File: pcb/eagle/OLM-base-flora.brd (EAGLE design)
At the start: 100 x 80 mm, 54 parts, among them CN1 MiniB USB, IC1 ATMEGA32U4-AU, IC2 LP2985-3.3v, IC3 DS1307, IC6 ENC28J60, T1 IRLML2246, U2 USD-SOCKETMICRO-SD-SOCKET-TAO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, X1 32.657k, X2A 25MHz, X2A1 25MHz, X3 8MHz

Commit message: added some details
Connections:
- removed net D0: U2.2
- removed net SCL: IC3.6, RCL.2
- removed net SDA: IC3.5, RDA.2
- net D2/SDA: now also IC3.5, RDA.2
- net D3/SCL: now also IC3.6, RCL.2
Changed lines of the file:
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@@
 <contactref element="IC1" pad="41"/>
-</signal>
-<signal name="D0">
-<contactref element="U2" pad="2"/>
 </signal>
 <signal name="RESET">
@@
 <contactref element="IC6" pad="9"/>
 </signal>
-<signal name="SDA">
-<contactref element="IC3" pad="5"/>
-<contactref element="RDA" pad="2"/>
-<wire x1="66.7766" y1="33.655" x2="66.99" y2="48.26" width="0" layer="19" extent="1-1"/>
-</signal>
-<signal name="SCL">
-<contactref element="IC3" pad="6"/>
-<contactref element="RCL" pad="2"/>
-<wire x1="66.7766" y1="32.385" x2="72.07" y2="40.64" width="0" layer="19" extent="1-1"/>
-</signal>
 <signal name="N$36">
 <contactref element="IC3" pad="3"/>
@@
 <signal name="D2/SDA">
 <contactref element="IC1" pad="19"/>
+<contactref element="IC3" pad="5"/>
+<contactref element="RDA" pad="2"/>
+<wire x1="66.99" y1="48.26" x2="81.61" y2="47.54" width="0" layer="19" extent="1-1"/>
+<wire x1="66.7766" y1="33.655" x2="66.99" y2="48.26" width="0" layer="19" extent="1-1"/>
 </signal>
 <signal name="D3/SCL">
 <contactref element="IC1" pad="18"/>
+<contactref element="IC3" pad="6"/>
+<contactref element="RCL" pad="2"/>
+<wire x1="72.07" y1="40.64" x2="80.81" y2="47.54" width="0" layer="19" extent="1-1"/>
+<wire x1="66.7766" y1="32.385" x2="72.07" y2="40.64" width="0" layer="19" extent="1-1"/>
 </signal>
 <signal name="D4/A6">

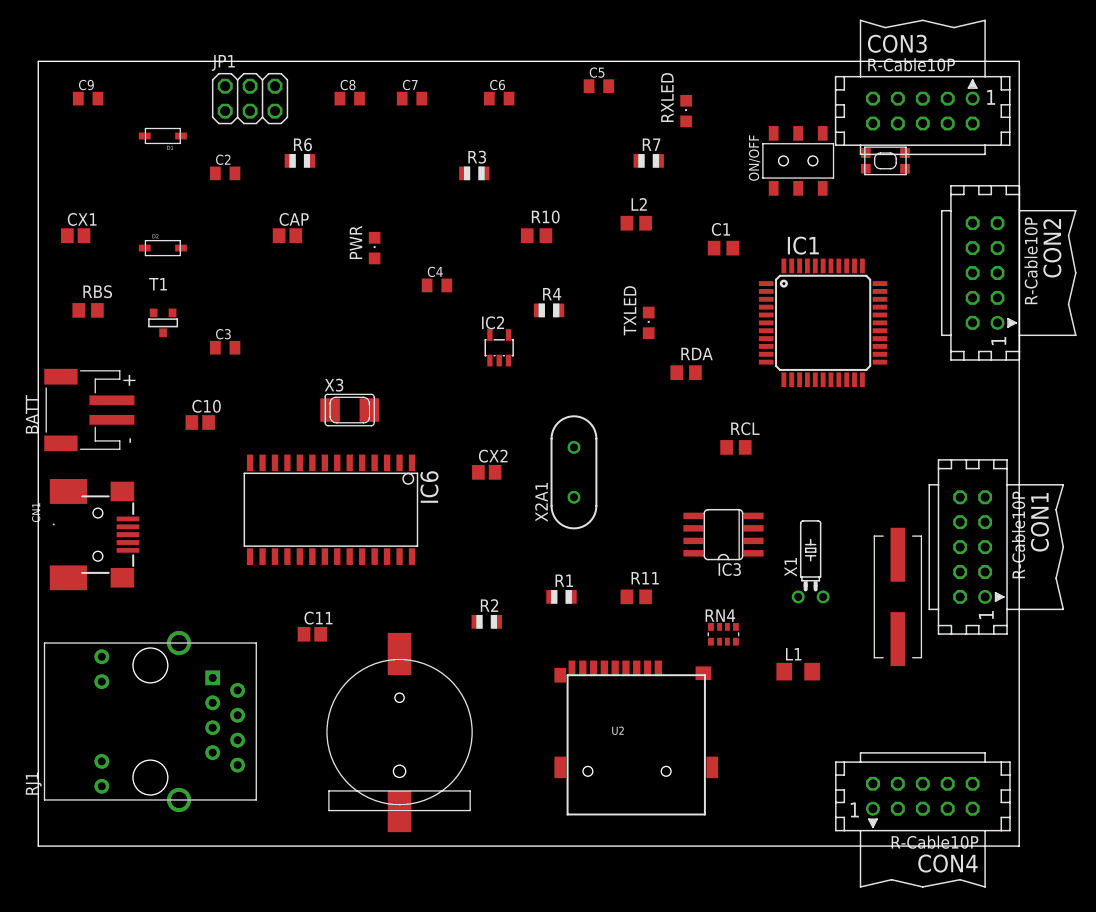
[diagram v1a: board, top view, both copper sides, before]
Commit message: made some changes
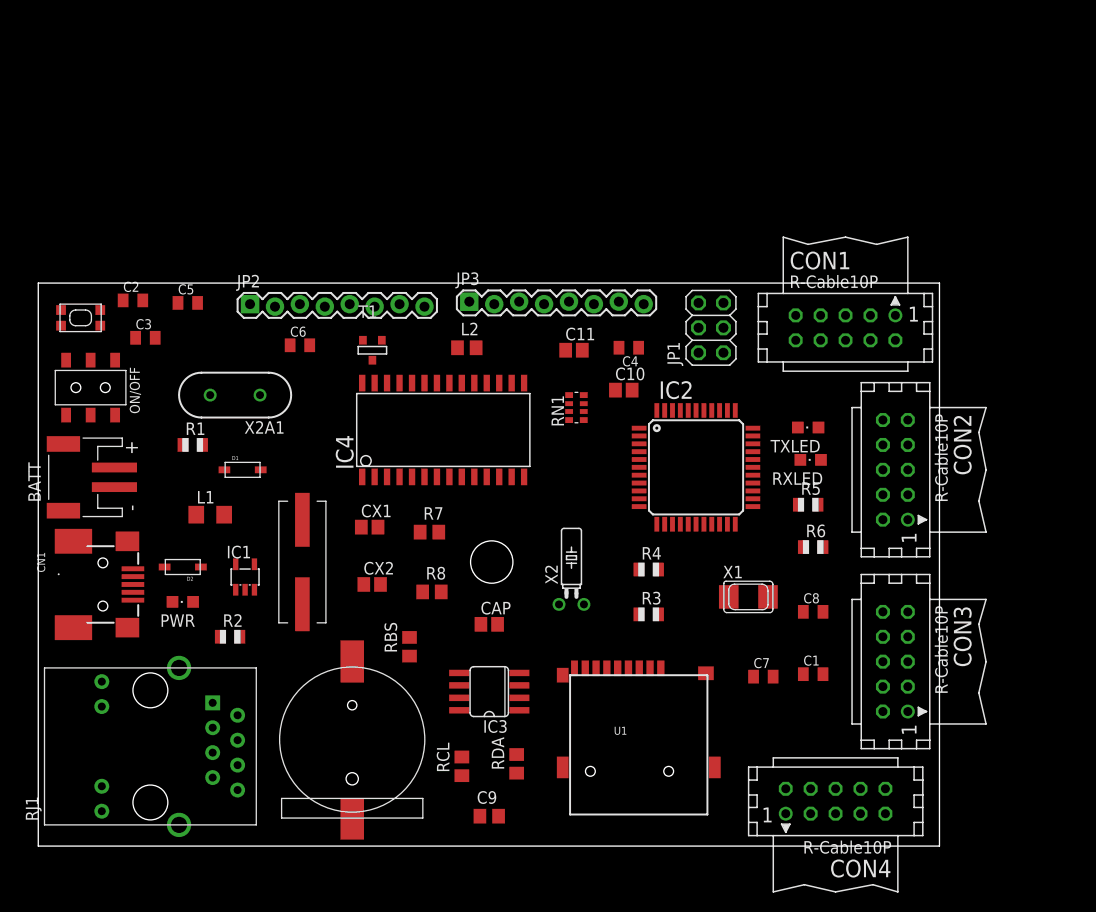
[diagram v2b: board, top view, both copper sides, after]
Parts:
- removed IC6: ENC28J60, SparkFun:SOIC28WLONG
- removed R10, R11: 330, rcl:R0805
- removed RN4: 49.9, resistor-dil:EXB38V
- removed U2: USD-SOCKETMICRO-SD-SOCKET-TAOBAO, SparkFunNew:MICRO-SD-SOCKET-TAOBAO
- removed X3: 8MHz, adaprog:NX5032
- added IC4: ENC28J60, SparkFun:SOIC28WLONG
- added JP2, JP3: (no value), SparkFun-Connectors:1X08_LOCK
- added R5: 1K, adafruit:R0805
- added R8: 330, rcl:R0805
- added RN1: 49.9, resistor-dil:EXB38V
- added U1: USD-SOCKETMICRO-SD-SOCKET-TAOBAO, SparkFunNew:MICRO-SD-SOCKET-TAOBAO
- added X2: 32.657k, crystal:TC26H
- C1: value 0.1u -> 10uF; device rcl:C0805 -> adafruit:C0805K
- C2, C3: value 18pF -> 10uF
- C7, C8: value 10uF -> 18pF
- C9: value 10uF -> 0.1u; device adafruit:C0805K -> rcl:C0805
- IC1: value ATMEGA32U4-AU -> LP2985-3.3v; device adaprog:TQFP44 -> adafruit:SOT23-5L
- IC2: value LP2985-3.3v -> ATMEGA32U4-AU; device adafruit:SOT23-5L -> adaprog:TQFP44
- R1: value 22 -> 10K
- R2: value 22 -> 470
- R3: value 470 -> 22
- R4: value 1K -> 22
- R7: value 10K -> 330; device adafruit:R0805 -> rcl:R0805
- X1: value 32.657k -> 8MHz; device crystal:TC26H -> adaprog:NX5032
- moved C9 83.8 mm to (46.0, 3.05)
- moved BOOT 83.6 mm to (4.32, 53.8)
- moved ON/OFF 75.7 mm to (5.33, 46.7), turned to 180 degrees
- moved C8 70.5 mm to (79.0, 23.9)
- moved C7 69.0 mm to (73.9, 17.3)
- moved R6 65.5 mm to (79.0, 30.5)
- moved IC1 64.4 mm to (21.1, 27.4)
- moved L1 62.0 mm to (17.5, 33.8)
- moved X2A 60.8 mm to (26.9, 29.0)
- moved CON3 56.2 mm to (87.4, 18.8), turned to 270 degrees
- moved JP1 52.5 mm to (68.6, 52.8), turned to 90 degrees
- moved R3 48.3 mm to (62.2, 23.6)
- moved RBS 47.4 mm to (37.8, 20.3), turned to 90 degrees
- moved C5 47.4 mm to (15.2, 55.4)
- moved CAP 44.6 mm to (46.0, 22.6)
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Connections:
- removed net AIO: CON1.4, CON2.4, CON3.4, CON4.4
- removed net DIO1: CON1.8, CON2.8, CON3.8, CON4.8
- removed net DIO2: CON1.9, CON2.9, CON3.9, CON4.9
- removed net DIO3: CON1.7, CON2.7, CON3.7, CON4.7
- new net A4/SDA: JP2.8
- new net A5/SCL: JP2.7
- new net D2: JP2.4
- new net D3/PWM: JP2.3
- new net E-CLK: JP2.6
- new net E-INT: JP2.5
- net +3V3: now also C2.1, C3.1, C4.1, C9.1, CON1.6, CON2.6, CON3.6, CON4.6, IC1.5, IC2.14, IC2.24, IC2.34, IC2.42, IC2.44, IC2.6, IC4.15, IC4.19, IC4.20, IC4.25, IC4.28, R2.2, U1.4; no longer C1.1, C6.1, C7.1, C8.1, IC1.14, IC1.24, IC1.34, IC1.42, IC1.44, IC1.6, IC2.5, IC6.15, IC6.19, IC6.20, IC6.25, IC6.28, R3.2, U2.4
- net +5V: now also C1.1, D2.A, IC2.7; no longer C9.1, D1.A, IC1.7
- net A0: now also CON1.4, CON3.4, IC2.36; no longer IC1.36
- net A1: now also CON1.2, CON3.2, IC2.37; no longer IC1.37
- net A2: now also CON2.4, CON4.4, IC2.38; no longer IC1.38
- net A3: now also CON2.2, CON4.2, IC2.39; no longer IC1.39
- net A4: now also IC2.40; no longer IC1.40
- net A5: now also IC2.41; no longer IC1.41
- net D0/RX: now also IC2.20, JP3.5; no longer IC1.20
- net D1/TX: now also IC2.21, JP3.4; no longer IC1.21
- net D2/SDA: now also IC2.19; no longer IC1.19
- net D3/SCL: now also IC2.18; no longer IC1.18
- net D4: now also IC4.9; no longer IC6.9
- net D4/A6: now also IC2.25; no longer IC1.25
- net D5*: now also CON1.9, CON3.9, IC2.31; no longer IC1.31
- net D6*/A8: now also IC2.27; no longer IC1.27
- net D7/AIN0: now also IC2.1; no longer IC1.1
- net GND: now also CON1.8, CON2.8, CON3.8, CON4.8, IC1.2, IC2.15, IC2.23, IC2.33, IC2.35, IC2.43, IC2.5, IC4.11, IC4.18, IC4.2, IC4.21, IC4.22, JP2.1, JP3.6, R5.2, U1.6; no longer CON1.6, CON2.6, CON3.6, CON4.6, IC1.15, IC1.23, IC1.33, IC1.35, IC1.43, IC1.5, IC2.2, IC6.11, IC6.18, IC6.2, IC6.21, IC6.22, R4.2, U2.6
- net IO10*/A11: now also CON1.7, CON3.7, IC2.30; no longer IC1.30
- net IO11*: now also IC2.12; no longer IC1.12
- net IO12*/A7: now also IC2.26; no longer IC1.26
- net IO13*: now also IC2.32; no longer IC1.32
- net IO8/A9: now also CON2.9, CON4.9, IC2.28; no longer IC1.28
- net IO9*/A10: now also CON2.7, CON4.7, IC2.29; no longer IC1.29
- net LEDA: now also R7.2; no longer R10.2
- net LEDB: now also R8.2; no longer R11.2
- net MISO: now also IC2.11, IC4.6, U1.7; no longer IC1.11, IC6.6, U2.7
- net MISO/D12: now also JP3.2
- net MOSI: now also IC2.10, IC4.7, U1.3; no longer IC1.10, IC6.7, U2.3
- net MOSI/D11: now also JP3.3
- net N$1: now also R2.1; no longer R3.1
- net N$11: now also R5.1; no longer R4.1
- net N$13: now also R1.1; no longer R7.1
- net N$2: now also R3.1; no longer R2.1
- net N$3: now also IC2.3, R4.2; no longer IC1.3, R1.2
- net N$34: now also IC4.27, R7.1; no longer IC6.27, R10.1
- net N$37: now also IC4.26, R8.1; no longer IC6.26, R11.1
- net N$39: now also IC4.1; no longer IC6.1
- net N$4: now also IC2.4, R3.2; no longer IC1.4, R2.2
- net N$41: now also IC4.24; no longer IC6.24
- net N$42: now also IC4.23; no longer IC6.23
- net N$47: now also X2.1; no longer X1.1
- net N$5: now also R4.1; no longer R1.1
- net N$50: now also X2.2; no longer X1.2
- net N$54: now also C10.2, RN1.5, RN1.6; no longer C11.2, RN4.5, RN4.6
- net N$59: now also IC4.14; no longer IC6.14
- net N$6: now also D1.C, R1.2; no longer D2.C, R7.2
- net N$7: now also D1.A; no longer D2.A
- net N$8: now also C7.1, IC2.17, X1.P$2; no longer C2.1, IC1.17, X3.P$2
- net N$9: now also C8.1, IC2.16, X1.P$1; no longer C3.1, IC1.16, X3.P$1
- net RD+: now also IC4.13, RN1.4; no longer IC6.13, RN4.4
- net RD-: now also IC4.12, RN1.3; no longer IC6.12, RN4.3
- net RESET: now also IC4.10; no longer IC6.10
- net RST: now also IC2.13; no longer IC1.13
- net RXLED/SS: now also IC2.8; no longer IC1.8
- net SCK: now also IC2.9, IC4.8, U1.5; no longer IC1.9, IC6.8, U2.5
- net SCK/D13: now also JP3.1
- net TCT: now also C11.2, RN1.7, RN1.8; no longer C10.2, RN4.7, RN4.8
- net TD+: now also IC4.17, RN1.2; no longer IC6.17, RN4.2
- net TD-: now also IC4.16, RN1.1; no longer IC6.16, RN4.1
- net TXLED: now also IC2.22; no longer IC1.22
- net VCC: now also C6.1, D2.C, IC1.1, IC1.3, JP2.2; no longer C4.1, CON1.10, CON2.10, CON3.10, CON4.10, D1.C, IC2.1, IC2.3
- net VIN: now also CON1.10, CON2.10, CON3.10, CON4.10, JP3.7, JP3.8; no longer CON1.2, CON2.2, CON3.2, CON4.2
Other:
- board size 100 x 80 mm -> 91.9 x 57.4 mm
